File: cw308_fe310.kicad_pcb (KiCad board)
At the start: 2 copper layers, 53.3 x 67.3 mm, 62 parts, among them J1 CW308T_CONNBOARD, J2 CrystalJumper, J3 10118193-0001LF, J4 Conn_02x05_Odd_Even, SW1 SW_Push, U1 IS25LP128, U2 SN74LVC1G07DBVR, U3 SN74LVC1G07DBVR, U4 FE310-G000, U5 FT2232HL-REEL, Y1 16Mhz, Y2 12MHz

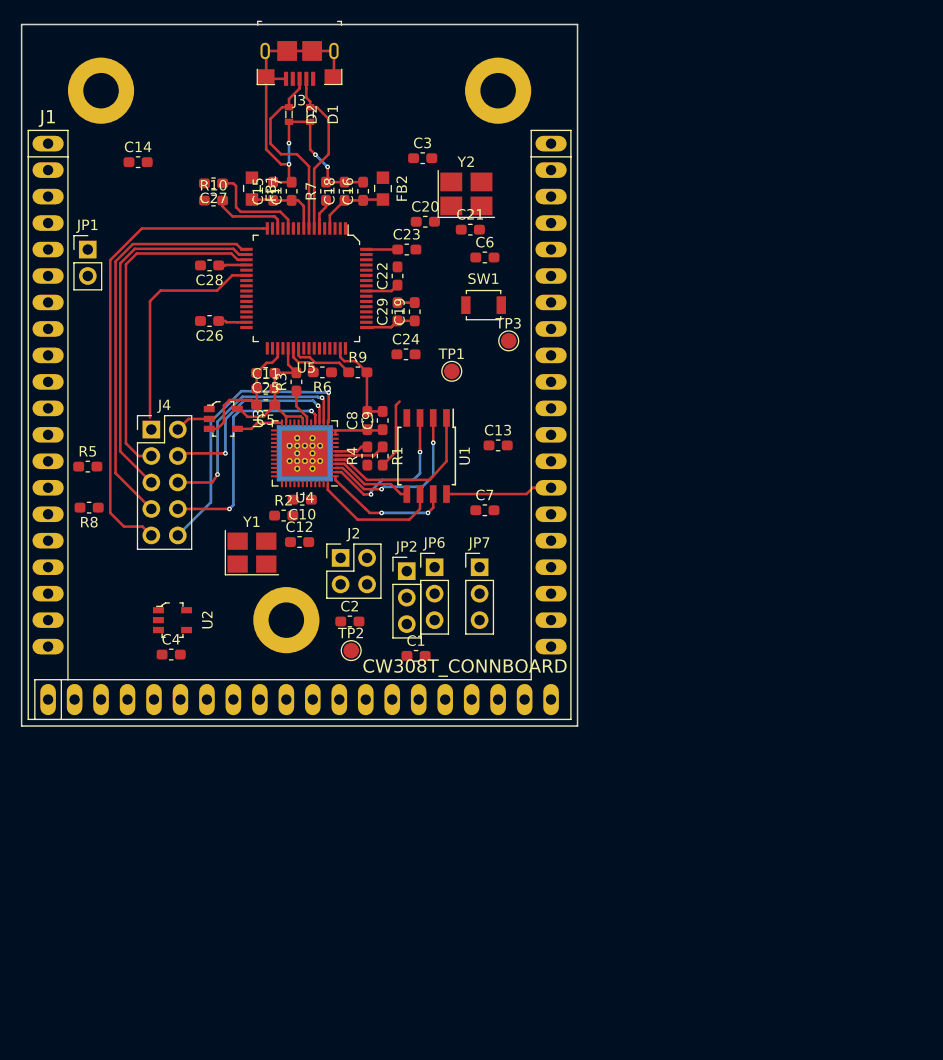
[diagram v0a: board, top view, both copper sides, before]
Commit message: simplified prototype ready
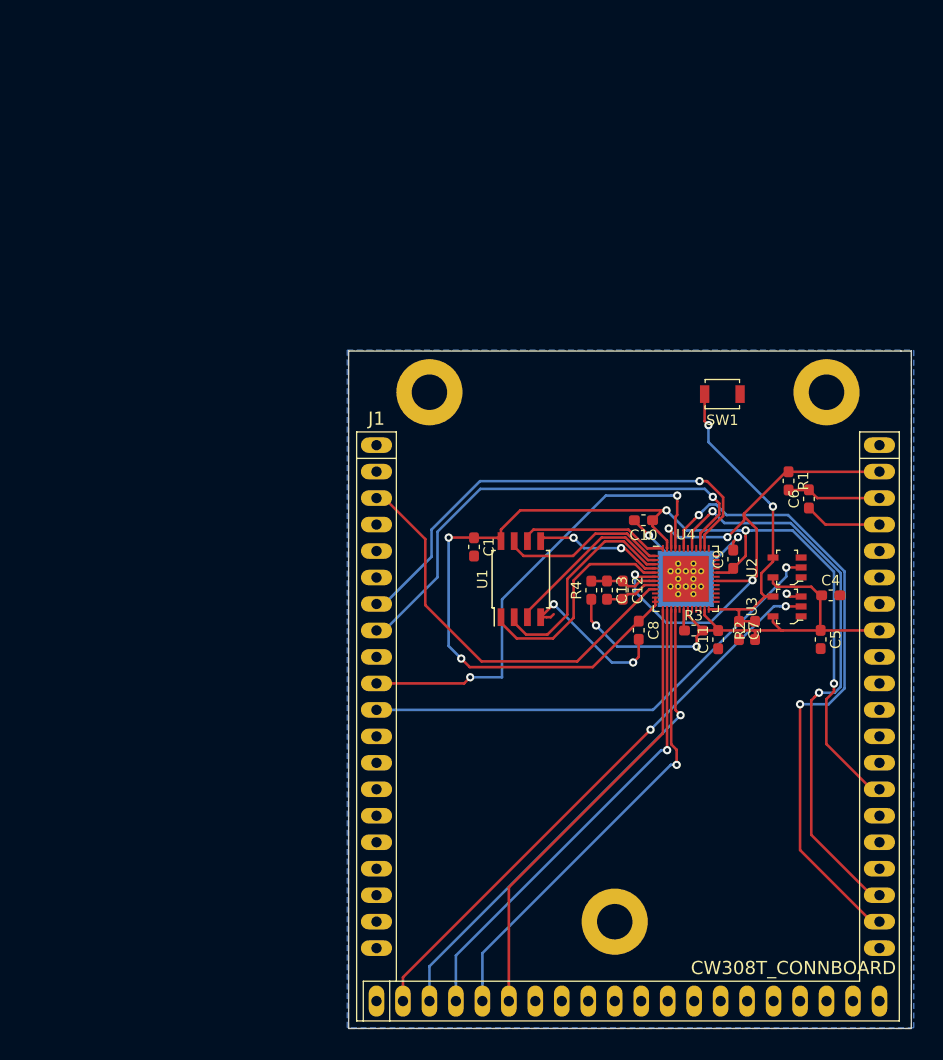
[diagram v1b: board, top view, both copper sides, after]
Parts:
- removed C14, C17, C18, C22, C23, C24, C25, C26, C27, C28, C29: 0.1uF, Capacitor_SMD:C_0603_1608Metric_Pad1.05x0.95mm_HandSolder
- removed C15, C16, C19: 4.7uF, Capacitor_SMD:C_0603_1608Metric_Pad1.05x0.95mm_HandSolder
- removed C2, C20, C21, C3: 12pF, Capacitor_SMD:C_0603_1608Metric_Pad1.05x0.95mm_HandSolder
- removed D1, D2: PGB1010603MR, digikey-footprints:0603
- removed FB1, FB2: MPZ2012S601AT000, digikey-footprints:0805
- removed J2: CrystalJumper, Connector_PinHeader_2.54mm:PinHeader_2x02_P2.54mm_Vertical
- removed J3: 10118193-0001LF, digikey-footprints:USB_Micro_B_Female_10118193-0001LF
- removed J4: Conn_02x05_Odd_Even, Connector_PinHeader_2.54mm:PinHeader_2x05_P2.54mm_Vertical
- removed JP1: Jumper, Connector_PinHeader_2.54mm:PinHeader_1x02_P2.54mm_Vertical
- removed JP2: Clock_Src_Sel, Connector_PinHeader_2.54mm:PinHeader_1x03_P2.54mm_Vertical
- removed JP6: TX_SEL, Connector_PinHeader_2.54mm:PinHeader_1x03_P2.54mm_Vertical
- removed JP7: RX_SEL, Connector_PinHeader_2.54mm:PinHeader_1x03_P2.54mm_Vertical
- removed R10, R5, R6, R8, R9: 1K, Resistor_SMD:R_0603_1608Metric_Pad1.05x0.95mm_HandSolder
- removed R7: 12K, Resistor_SMD:R_0603_1608Metric_Pad1.05x0.95mm_HandSolder
- removed TP1, TP2, TP3: TestPoint, TestPoint:TestPoint_Pad_D1.5mm
- removed U5: FT2232HL-REEL, digikey-footprints:LQFP-64_10x10mm
- removed Y1: 16Mhz, Oscillator:Oscillator_SMD_Abracon_ASE-4Pin_3.2x2.5mm_HandSoldering
- removed Y2: 12MHz, Crystal:Crystal_SMD_TXC_7M-4Pin_3.2x2.5mm_HandSoldering
- moved C4 63.5 mm to (165.3, 81.4)
- moved U2 59.2 mm to (161.1, 78.8), turned to 90 degrees
- moved C5 57.8 mm to (164.3, 85.7), turned to 270 degrees
- moved U3 57.0 mm to (161.1, 82.5), turned to 90 degrees
- moved C11 49.6 mm to (154.5, 85.7), turned to 90 degrees
- moved R2 46.5 mm to (158.0, 84.8), turned to 90 degrees
- moved R3 45.0 mm to (152.1, 84.8), turned to 0 degrees
- moved J1 42.8 mm to (121.7, 67.0)
- moved R1 39.0 mm to (161.2, 70.5)
- moved C6 38.8 mm to (163.2, 72.2), turned to 90 degrees
- moved U4 38.5 mm to (151.4, 79.9), turned to 0 degrees
- moved C9 36.2 mm to (155.9, 78.0)
- moved C8 32.9 mm to (146.8, 84.8), turned to 270 degrees
- moved C10 32.8 mm to (147.3, 74.2)
- moved C12 31.3 mm to (145.3, 80.9), turned to 270 degrees
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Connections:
- J1 pad B2: Net-(J1-PadB2) -> JTAG_TRST
- J1 pad B3: Net-(J1-PadB3) -> JTAG_TDI
- J1 pad B4: Net-(J1-PadB4) -> JTAG_TDO
- J1 pad B5: Net-(J1-PadB5) -> JTAG_TMS
- J1 pad B6: Net-(J1-PadB6) -> JTAG_TCK
- U4 pad 10: XTAL_XO -> Net-(U4-Pad10)
- U4 pad 38: RX -> GPIO1
- U4 pad 39: TX -> GPIO2
- U4 pad 9: XTAL_XI -> CLKIN
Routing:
- net +3V3: track 23.9 -> 110.4 mm, vias 0 -> 5
- net LED2: track 0.00 -> 61.4 mm, vias 0 -> 2
- net LED1: track 0.00 -> 55.2 mm, vias 0 -> 2
- net JTAG_TRST: track 3.44 -> 55.2 mm, vias 0 -> 2
- net VCC_CLEAN: track 4.88 -> 54.0 mm, vias 0 -> 4
- net UFO.RST: track 0.00 -> 46.9 mm, vias 0 -> 1
- net GPIO2: track 0.00 -> 46.7 mm, vias 0 -> 1
- net GPIO1: track 0.00 -> 45.9 mm, vias 0 -> 1
- net GPIO4: track 0.00 -> 45.8 mm, vias 0 -> 2
- net FTDI.JTAG_TCK: track 45.4 -> 0.00 mm
- net CLKIN: track 0.00 -> 39.8 mm
- net FTDI.JTAG_TDI: track 38.6 -> 0.00 mm
- net FTDI.JTAG_TDO: track 35.2 -> 0.00 mm
- net FTDI.JTAG_TMS: track 32.4 -> 0.00 mm
- net Net-(C7-Pad1): track 3.95 -> 32.2 mm, vias 0 -> 2
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- added copper zone on B.Cu, net GND
- added copper zone on F.Cu, net GND
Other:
- board size 53.3 x 67.3 mm -> 54 x 65 mm
- net class Default: clearance 0.127 -> 0.12
- rule pad_to_mask_clearance: 0.051 -> 0
- rule trace_clearance: 0.127 -> 0.12
- rule trace_min: 0.0889 -> 0.2
- rule via_min_drill: 0.2 -> 0.3
- rule via_min_size: 0.45 -> 0.4

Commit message: revision 0.1
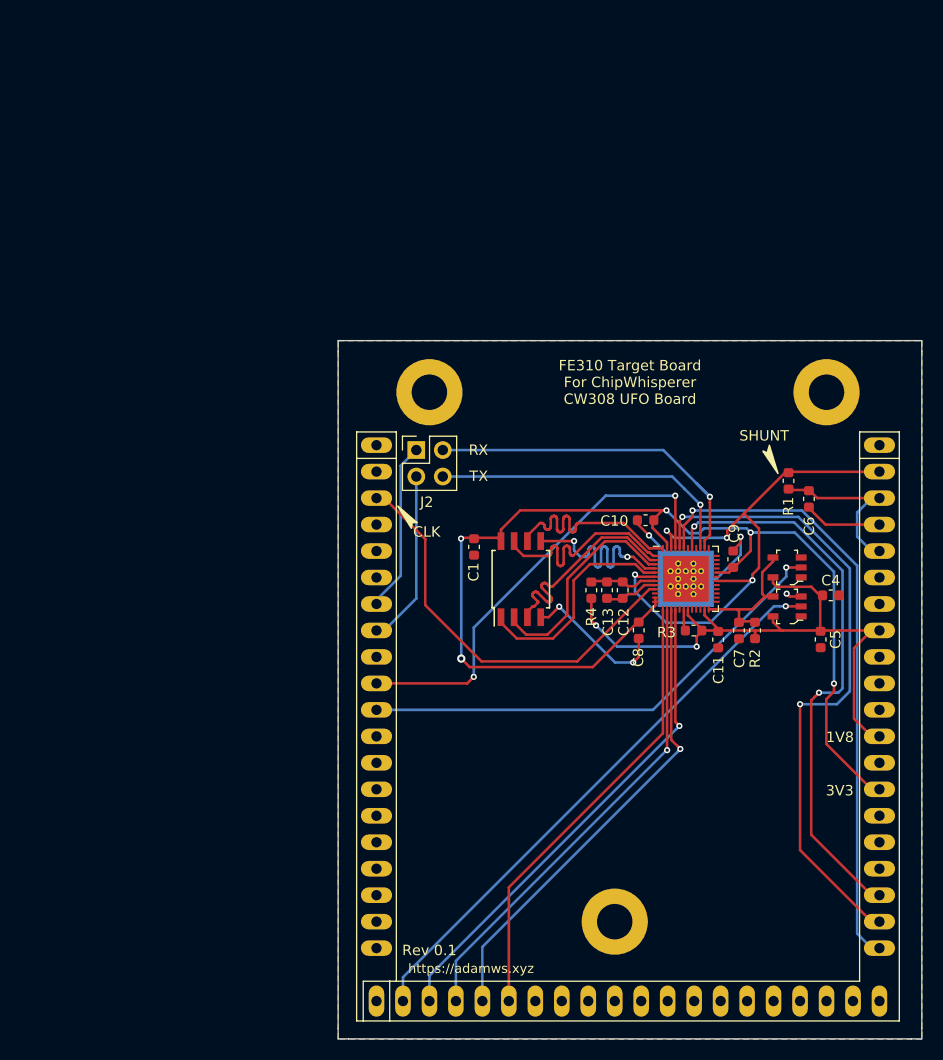
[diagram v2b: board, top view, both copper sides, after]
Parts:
- removed SW1: SW_Push, Button_Switch_SMD:SW_SPST_B3U-1000P
- added G***: LOGO, cw308_fe310:logo, B.Cu at (155.2, 107.5)
- added J2: SerialSel, Connector_PinHeader_2.54mm:PinHeader_2x02_P2.54mm_Vertical, F.Cu at (125.5, 67.5)
- C1, C10, C11, C12, C13, C4, C5, C6, C7, C8, C9: footprint Capacitor_SMD:C_0603_1608Metric_Pad1.05x0.95mm_HandSolder -> Capacitor_SMD:C_0603_1608Metric
- R1, R2, R3, R4: footprint Resistor_SMD:R_0603_1608Metric_Pad1.05x0.95mm_HandSolder -> Resistor_SMD:R_0603_1608Metric
- moved C10 0.21 mm to (147.5, 74.2)
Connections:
- J1 pad C20: LED2 -> LED3
- U4 pad 38: GPIO1 -> RX
- U4 pad 39: GPIO2 -> TX
- U4 pad 43: LED2 -> LED3
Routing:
- net LED3: track 0.00 -> 60.0 mm, vias 0 -> 1
- net RX: track 0.00 -> 34.5 mm, vias 0 -> 1
- net TX: track 0.00 -> 30.0 mm, vias 0 -> 1
- net GPIO2: track 46.7 -> 16.8 mm, vias 1 -> 0
- net GPIO1: track 45.9 -> 16.4 mm, vias 1 -> 0
- net Net-(C7-Pad1): track 32.2 -> 13.7 mm, vias 2 -> 0
- net +1V8: track 48.7 -> 61.8 mm
- net FLASH_IO0: track 12.4 -> 21.0 mm
- net Net-(C6-Pad2): track 9.07 -> 16.8 mm
- net FLASH_SCK: track 14.5 -> 21.0 mm
- net FLASH_IO3: track 16.2 -> 21.0 mm
- net FLASH_IO2: track 16.6 -> 21.2 mm
- net GPIO4: track 45.8 -> 44.0 mm
- net +3V3: track 110.4 -> 109.0 mm
- net LED2: track 61.4 -> 62.8 mm
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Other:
- board size 54 x 65 mm -> 56 x 67 mm
- board text added: "1V8"
- board text added: "3V3"
- board text added: "CLK"
- board text added: "FE310 Target Board For ChipWhisperer CW308 UFO Board"
- board text added: "R"
- board text added: "Rev 0.1"
- board text added: "SHUNT"
- board text added: "T"
- board text added: "X"
- board text added: "https://adamws.xyz"
